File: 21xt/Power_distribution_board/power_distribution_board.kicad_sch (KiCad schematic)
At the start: 28 parts, among them IC1 LM74700QDBVRQ1, IC2 LM74700QDBVRQ1, IC3 LTC2959IDDB#TRMPBF, IC4 INA180A1IDBVR, IC5 TLV76150DCYR, J2 Conn_01x02, J3 Conn_01x02, J4 Conn_01x02, Q1 NVMFWS2D1N08XT1G, Q2 NVMFWS2D1N08XT1G, U1 esp32 c6 xiao

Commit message: aaaa
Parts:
- R1: footprint 21xt_footprints:R_0603_1608Metric_Pad0.98x0.95mm_HandSolder -> hi:RESC_WSHM2818R0150FEA
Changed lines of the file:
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@@
 			)
 		)
-		(property "Footprint" "21xt_footprints:R_0603_1608Metric_Pad0.98x0.95mm_HandSolder"
+		(property "Footprint" "hi:RESC_WSHM2818R0150FEA"
 			(at 220.98 137.668 90)
 			(effects

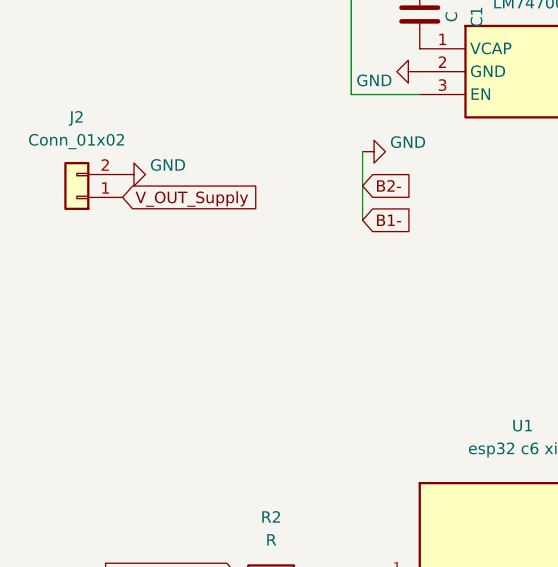
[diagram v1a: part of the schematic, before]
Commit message: aaa
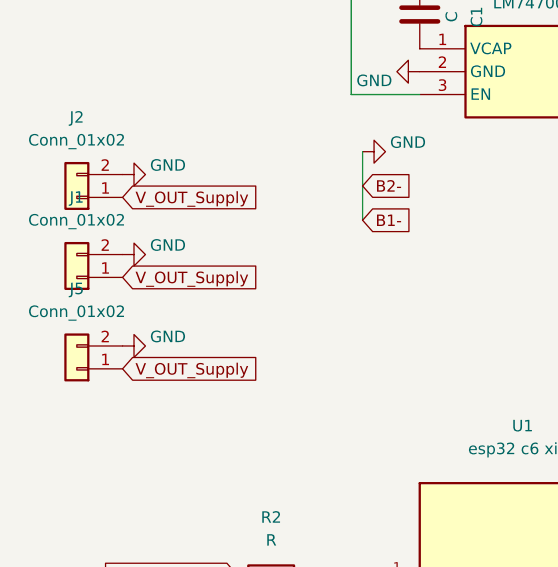
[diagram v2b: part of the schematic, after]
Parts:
- added J1, J5: Conn_01x02, 21xt_footprints:Deans Connector Female, symbol Connector_Generic:Conn_01x02
- J2: footprint 21xt_footprints:Deans Connector Male -> 21xt_footprints:Deans Connector Female
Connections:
- net GND: now also J1.2 (Pin_2), J5.2 (Pin_2)
- net V_OUT_Supply: now also J1.1 (Pin_1), J5.1 (Pin_1)
